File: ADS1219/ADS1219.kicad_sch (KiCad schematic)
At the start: 26 parts, among them J1 Conn_01x04, J2 Conn_01x06, J3 Conn_01x04, U1 ADS1219IPW

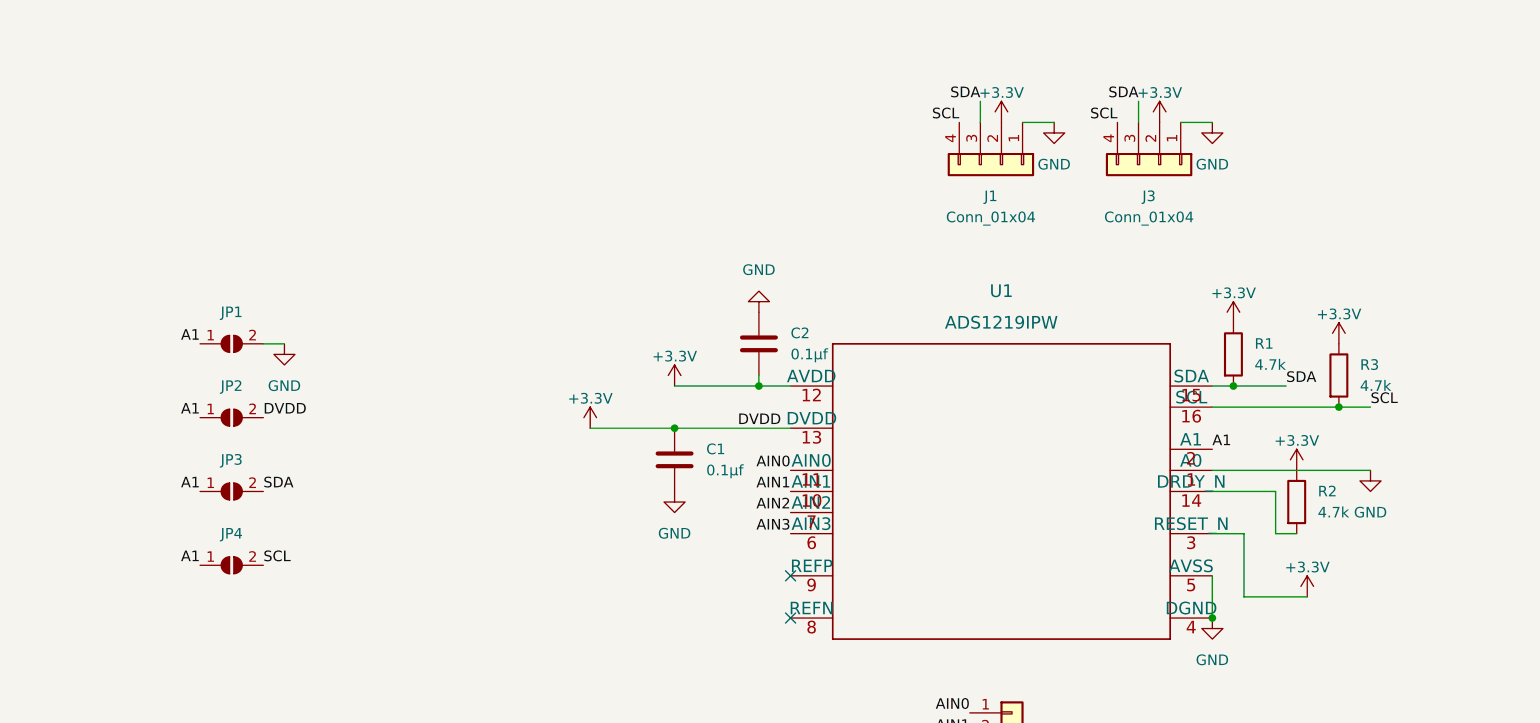
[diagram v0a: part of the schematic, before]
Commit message: Adding slider for address programming
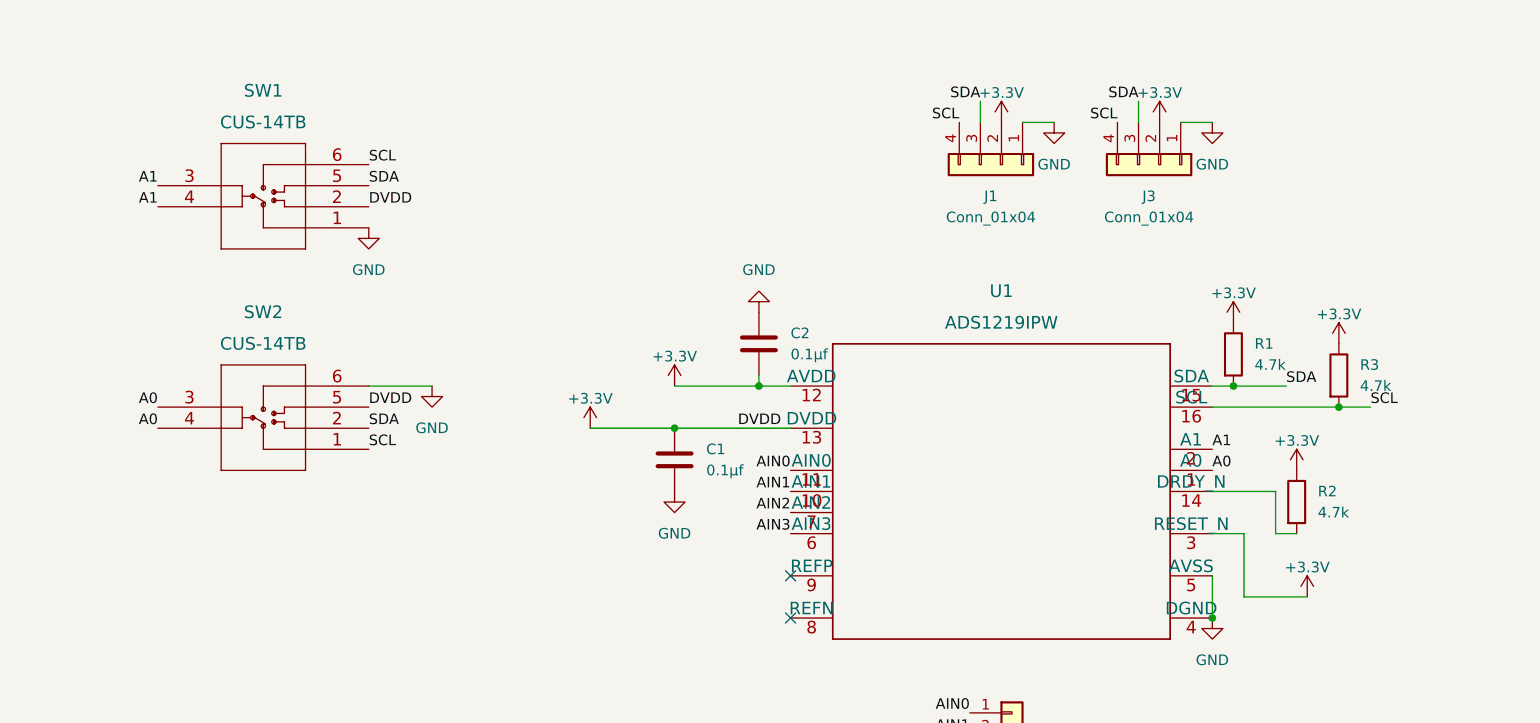
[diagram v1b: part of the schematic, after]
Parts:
- removed JP1, JP2, JP3, JP4: SolderJumper_2_Open, Jumper:SolderJumper-2_P1.3mm_Open_TrianglePad1.0x1.5mm, symbol Jumper:SolderJumper_2_Open
- added SW1, SW2: CUS-14TB, ul_CUS-14TB:CUS-14TB, symbol ul_CUS-14TB:CUS-14TB
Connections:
- net +3.3V: now also SW1.2, SW2.5
- net A1: now also SW1.3, SW1.4
- net GND: now also SW1.1, SW2.6; no longer U1.1 (A0)
- net SCL: now also SW1.6, SW2.1
- net SDA: now also SW1.5, SW2.2
- new net A0: SW2.3, SW2.4, U1.1 (A0)

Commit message: Revert "Adding slider for address programming"
This reverts commit 487b6004aa2a68d069b1c4fba08261144dd1fb57.
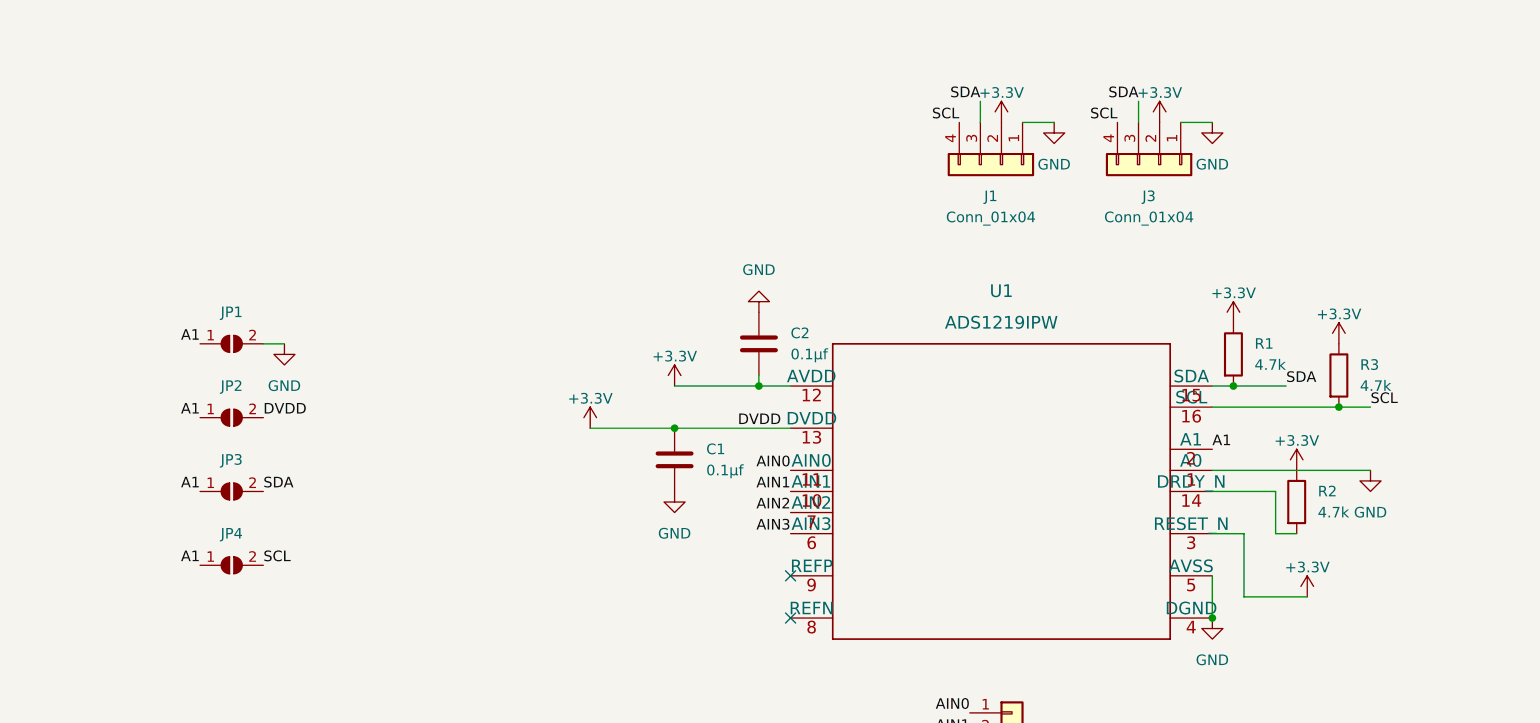
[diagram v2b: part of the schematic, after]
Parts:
- removed SW1, SW2: CUS-14TB, ul_CUS-14TB:CUS-14TB, symbol ul_CUS-14TB:CUS-14TB
- added JP1, JP2, JP3, JP4: SolderJumper_2_Open, Jumper:SolderJumper-2_P1.3mm_Open_TrianglePad1.0x1.5mm, symbol Jumper:SolderJumper_2_Open
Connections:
- net A0 is gone; now on net GND: U1.1 (A0)
- net +3.3V: now also JP2.2 (B)
- net A1: now also JP1.1 (A), JP2.1 (A), JP3.1 (A), JP4.1 (A)
- net GND: now also JP1.2 (B)
- net SCL: now also JP4.2 (B)
- net SDA: now also JP3.2 (B)
